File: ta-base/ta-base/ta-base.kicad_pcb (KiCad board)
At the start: 2 copper layers, 64 x 58 mm, 15 parts, among them P1 Gnd_Screws, SW1 SW_SPDT, SW2 SW_SPDT, U1 BSB008NE2LXXUMA1, U2 burn_wire

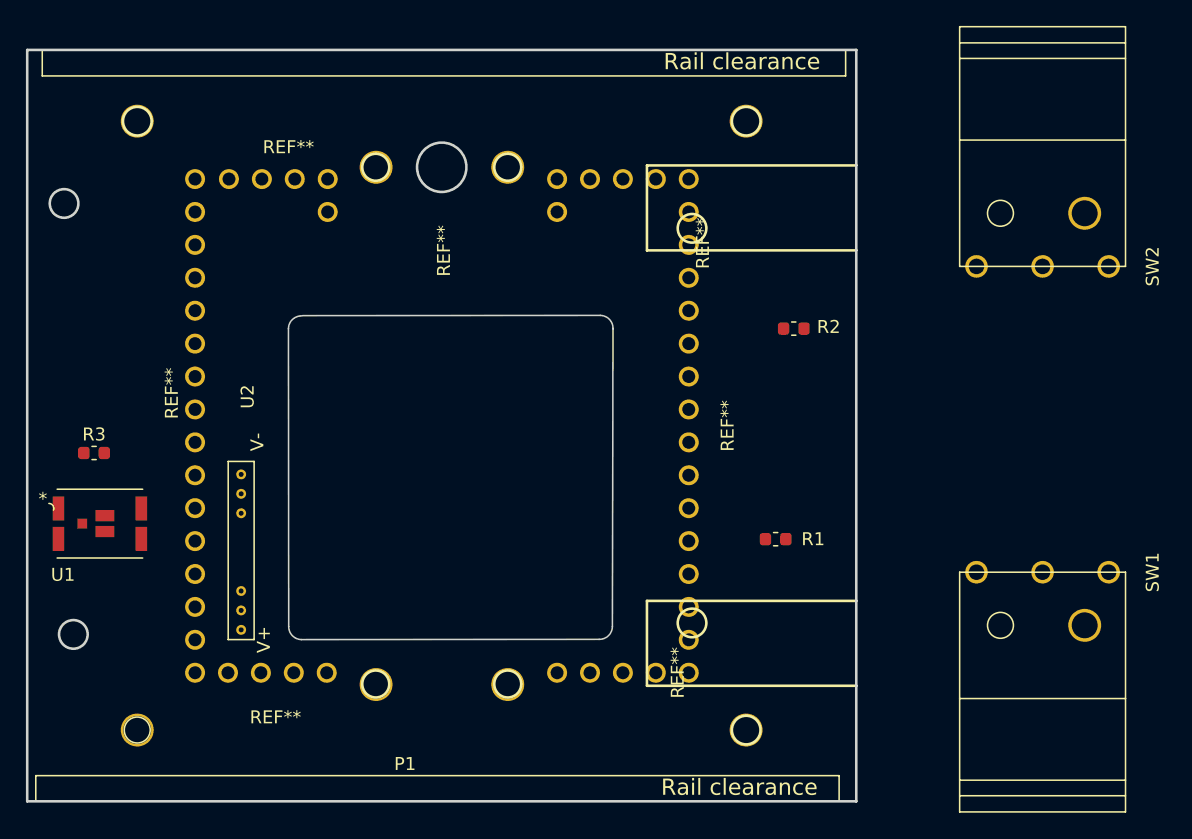
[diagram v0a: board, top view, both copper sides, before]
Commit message: finalized place and route
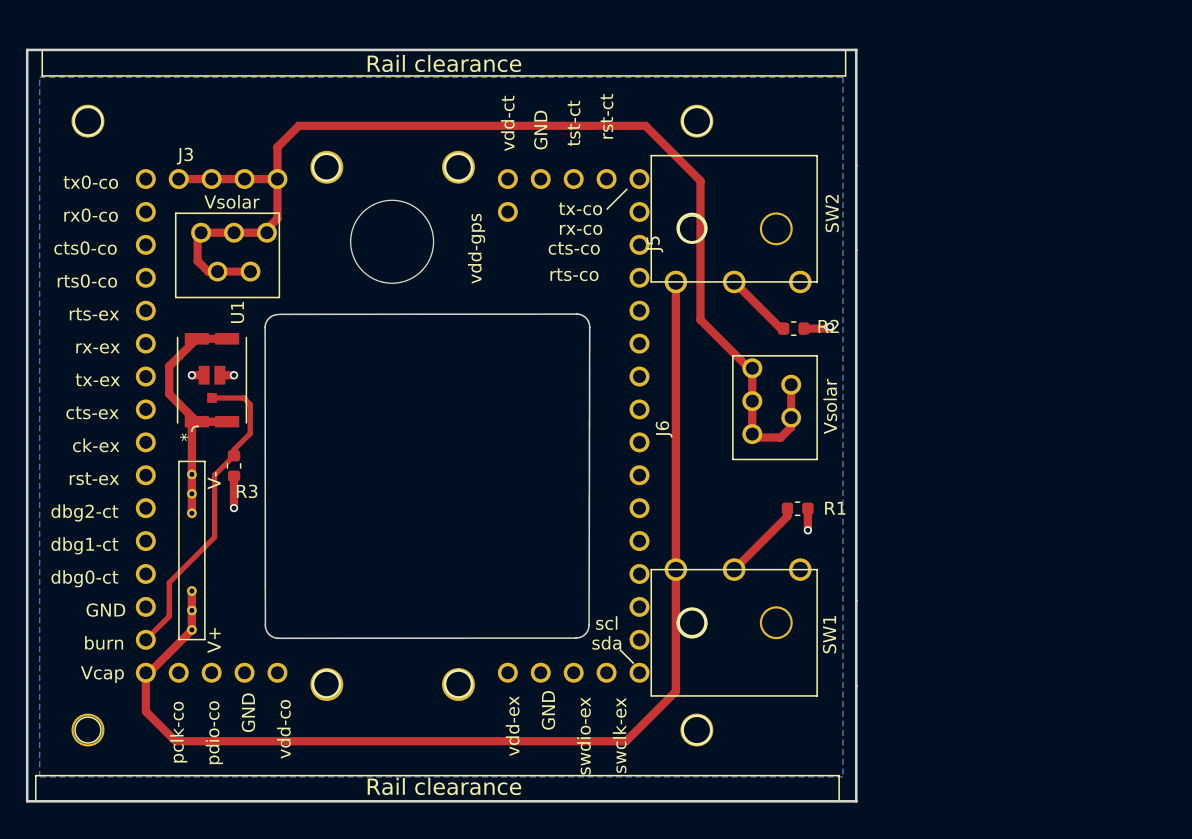
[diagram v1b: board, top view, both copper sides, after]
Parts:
- removed the REF** at (183.9, 85.5)
- removed the REF** at (155.9, 85.5)
- removed the REF** at (182.5, 123.6)
- removed the REF** at (157.1, 123.6)
- removed the REF** at (188.9, 104.5)
- removed the REF** at (150.8, 104.5)
- removed the REF** at (169.8, 84.5)
- added J1: PinSocket_16_base, ta-base:PinSocket_1x16_TartanArtibeus_base_cpy, F.Cu at (147.0, 104.5)
- added J2: PinSocket_4_base, ta-base:PinSocket_1x4_TartanArtibeus_base_cpy, F.Cu at (178.7, 123.6)
- added J3: PinSocket_4_base, ta-base:PinSocket_1x4_TartanArtibeus_base_cpy, F.Cu at (153.3, 85.5)
- added J4: PinSocket_4_base, ta-base:PinSocket_1x4_TartanArtibeus_base_cpy, F.Cu at (153.3, 123.6)
- added J5: PinSocket_5_base, ta-base:PinSocket_1x5_right_TartanArtibeus_base_cpy, F.Cu at (180.1, 85.5)
- added J6: PinSocket_16_base, ta-base:PinSocket_1x16_TartanArtibeus_base_cpy, F.Cu at (185.1, 104.5)
- added J7: PinSocket_5_base, ta-base:solar_internal, F.Cu at (153.8, 89.6)
- added J8: PinSocket_5_base, ta-base:solar_internal, F.Cu at (193.8, 102.6)
- added P2: Gnd_standoffs, ta-base:MountingHoles_TartanArtibeus_base_cpy, F.Cu at (166.0, 84.5)
- added REF**: MountingHole_6.4mm_M6, MountingHole:MountingHole_6.4mm_M6, F.Cu at (166.0, 90.3)
- U1: value BSB008NE2LXXUMA1 -> TRANS_BSB008NE2LXXUMA1_INF
- moved SW2 23.8 mm to (192.4, 93.4)
- moved SW1 23.8 mm to (192.4, 115.6)
- moved U1 14.0 mm to (152.1, 101.0), turned to 90 degrees
- moved R3 10.8 mm to (153.8, 107.6), turned to 270 degrees
- moved P1 3.80 mm to (142.5, 128.0)
- moved U2 3.80 mm to (150.6, 111.2)
- moved R1 2.90 mm to (197.3, 110.9)
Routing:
- net /V_solar: track 0.00 -> 89.0 mm
- net /Vcap: track 0.00 -> 86.0 mm
- net /BURN_SIG: track 0.00 -> 24.7 mm
- net Net-(U1-Pad4): track 0.00 -> 20.8 mm
- net GND: track 0.00 -> 8.37 mm, vias 0 -> 5
- net Net-(R1-Pad2): track 0.00 -> 6.40 mm
- net Net-(R2-Pad2): track 0.00 -> 5.30 mm
- added copper zone on B.Cu, net GND
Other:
- outline, holes or cut-outs redrawn
- board text added: "GND"
- board text added: "Vcap"
- board text added: "Vsolar"
- board text added: "burn"
- board text added: "ck-ex"
- board text added: "cts-co"
- board text added: "cts-ex"
- board text added: "cts0-co"
- board text added: "dbg0-ct"
- board text added: "dbg1-ct"
- board text added: "dbg2-ct"
- board text added: "pclk-co"
- board text added: "pdio-co"
- board text added: "rst-ct"
- board text added: "rst-ex"
- board text added: "rts-co"
- board text added: "rts-ex"
- board text added: "rts0-co"
- board text added: "rx-co"
- board text added: "rx-ex"
- board text added: "rx0-co"
- board text added: "scl"
- board text added: "sda"
- board text added: "swclk-ex"
- board text added: "swdio-ex"
- board text added: "tst-ct"
- board text added: "tx-co"
- board text added: "tx-ex"
- board text added: "tx0-co"
- board text added: "vdd-co"
- board text added: "vdd-ct"
- board text added: "vdd-ex"
- board text added: "vdd-gps"
